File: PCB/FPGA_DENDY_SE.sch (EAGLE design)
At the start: 138 parts, among them CN1 DENDY60PINSLOT, J1 NTSC/PAL, J2 DENDY, Q1 14.318 MHz, Q2 17.734 MHz, U1 EP1C3T100C8N, U10 OPA2134U, U11 SN74LVC2G34DBVR, U12 THS7314DR, U13 74LS373WMSO20, U14 SN74LVC1G125DBVR, U15 74LVC1G04GV, U16 SN74LVC1G3157, U2 EPCS4, U3 SN74LVC8T245, U4 SN74LVC8T245, U5 SN74LVC1G240DBVR, U6 SN74LVC1G240DBVR, U7 SN74LVC1G240DBVR, U8 SN74LVC1G240DBVR, X1 057-010-1

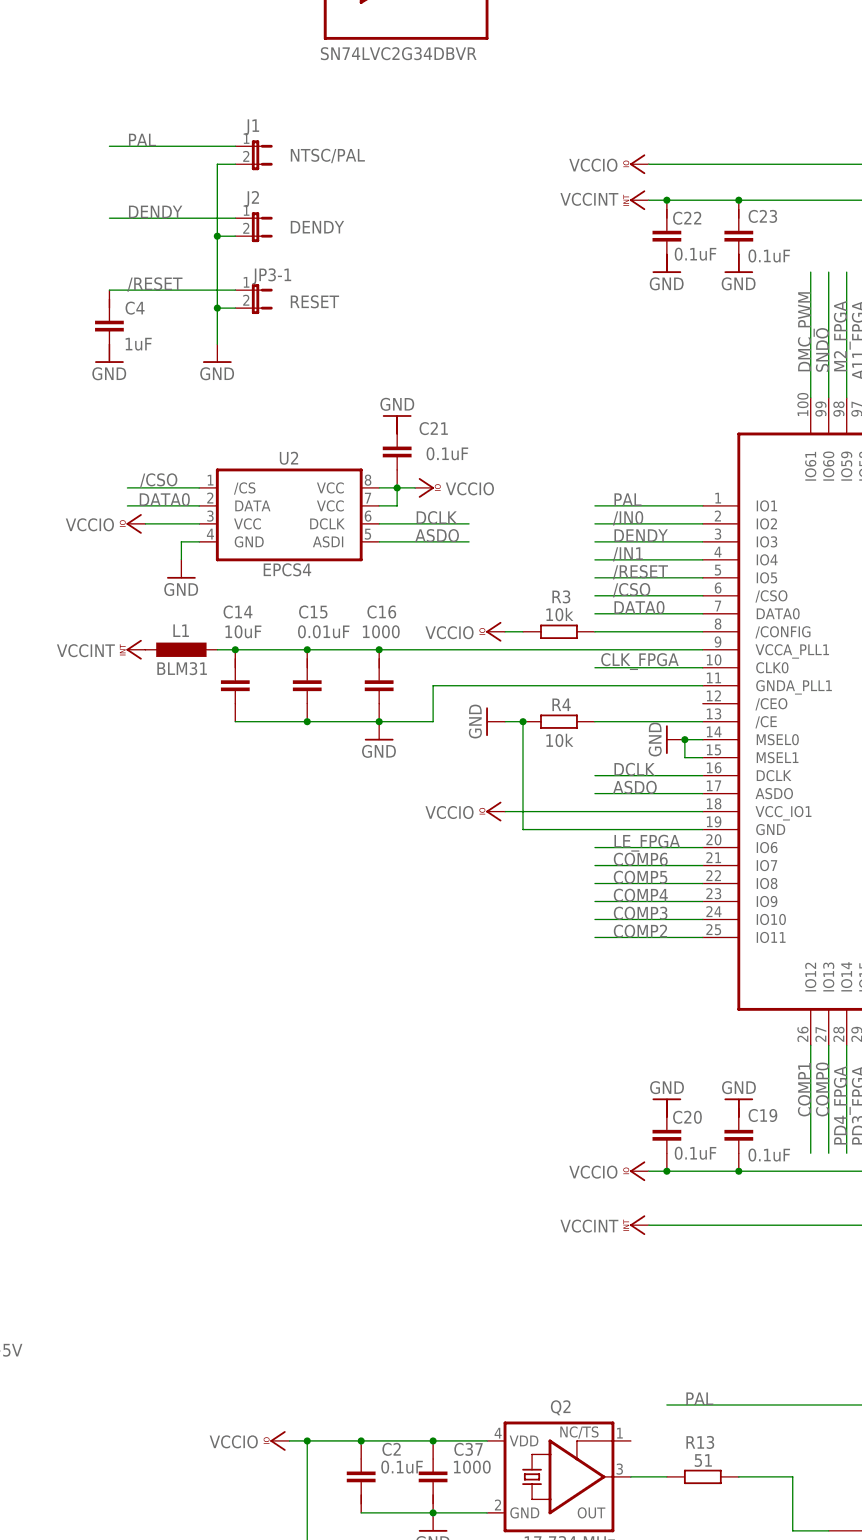
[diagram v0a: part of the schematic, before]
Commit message: Add files via upload
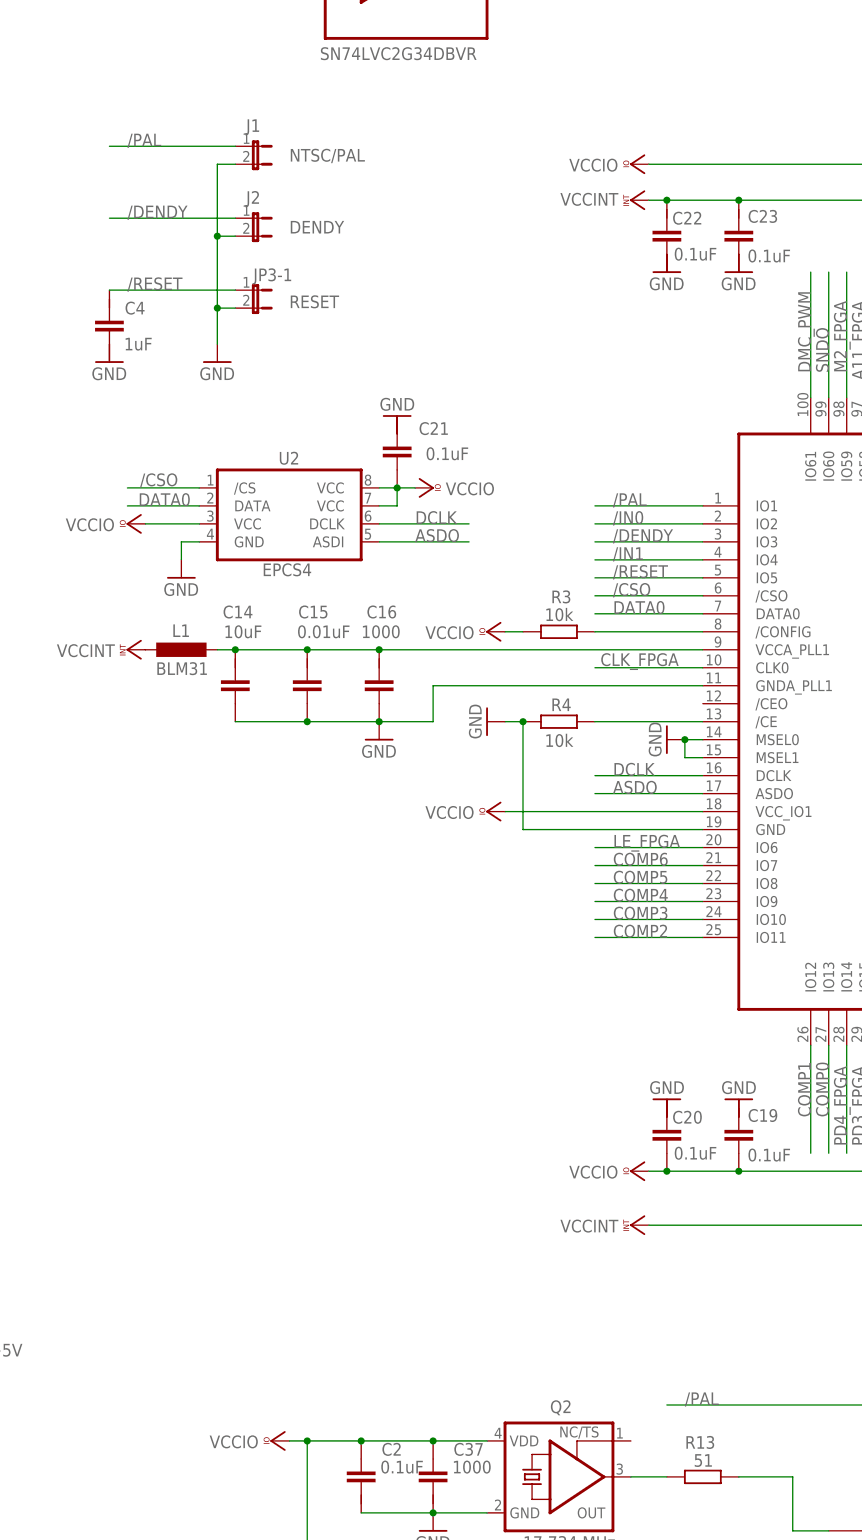
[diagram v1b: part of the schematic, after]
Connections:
- net DENDY renamed /DENDY
- net PAL renamed /PAL
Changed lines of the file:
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@@
-</segment>
-</net>
-<net name="DENDY" class="0">
-<segment>
-<pinref part="J2" gate="A" pin="1"/>
-<wire x1="-111.76" y1="68.58" x2="-129.54" y2="68.58" width="0.1524" layer="91"/>
-<label x="-127" y="68.58" size="1.778" layer="95"/>
-</segment>
-<segment>
-<wire x1="-45.72" y1="22.86" x2="-60.96" y2="22.86" width="0.1524" layer="91"/>
-<label x="-58.42" y="22.86" size="1.778" layer="95"/>
-<pinref part="U1" gate="G$1" pin="IO3"/>
 </segment>
 </net>
@@
 <pinref part="Q2" gate="G$1" pin="OUT"/>
 <wire x1="-50.8" y1="-109.22" x2="-55.88" y2="-109.22" width="0.1524" layer="91"/>
-</segment>
-</net>
-<net name="PAL" class="0">
-<segment>
-<pinref part="J1" gate="A" pin="1"/>
-<wire x1="-111.76" y1="78.74" x2="-129.54" y2="78.74" width="0.1524" layer="91"/>
-<label x="-127" y="78.74" size="1.778" layer="95"/>
-</segment>
-<segment>
-<wire x1="-45.72" y1="27.94" x2="-60.96" y2="27.94" width="0.1524" layer="91"/>
-<label x="-58.42" y="27.94" size="1.778" layer="95"/>
-<pinref part="U1" gate="G$1" pin="IO1"/>
-</segment>
-<segment>
-<wire x1="-17.78" y1="-99.06" x2="-50.8" y2="-99.06" width="0.1524" layer="91"/>
-<label x="-48.26" y="-99.06" size="1.778" layer="95"/>
-<pinref part="U16" gate="G$1" pin="S"/>
-<wire x1="-17.78" y1="-99.06" x2="-17.78" y2="-106.68" width="0.1524" layer="91"/>
 </segment>
 </net>
@@
 </segment>
 </net>
+<net name="/PAL" class="0">
+<segment>
+<pinref part="J1" gate="A" pin="1"/>
+<wire x1="-111.76" y1="78.74" x2="-129.54" y2="78.74" width="0.1524" layer="91"/>
+<label x="-127" y="78.74" size="1.778" layer="95"/>
+</segment>
+<segment>
+<wire x1="-45.72" y1="27.94" x2="-60.96" y2="27.94" width="0.1524" layer="91"/>
+<label x="-58.42" y="27.94" size="1.778" layer="95"/>
+<pinref part="U1" gate="G$1" pin="IO1"/>
+</segment>
+<segment>
+<wire x1="-17.78" y1="-99.06" x2="-50.8" y2="-99.06" width="0.1524" layer="91"/>
+<label x="-48.26" y="-99.06" size="1.778" layer="95"/>
+<pinref part="U16" gate="G$1" pin="S"/>
+<wire x1="-17.78" y1="-99.06" x2="-17.78" y2="-106.68" width="0.1524" layer="91"/>
+</segment>
+</net>
+<net name="/DENDY" class="0">
+<segment>
+<pinref part="J2" gate="A" pin="1"/>
+<wire x1="-111.76" y1="68.58" x2="-129.54" y2="68.58" width="0.1524" layer="91"/>
+<label x="-127" y="68.58" size="1.778" layer="95"/>
+</segment>
+<segment>
+<wire x1="-45.72" y1="22.86" x2="-60.96" y2="22.86" width="0.1524" layer="91"/>
+<label x="-58.42" y="22.86" size="1.778" layer="95"/>
+<pinref part="U1" gate="G$1" pin="IO3"/>
+</segment>
+</net>

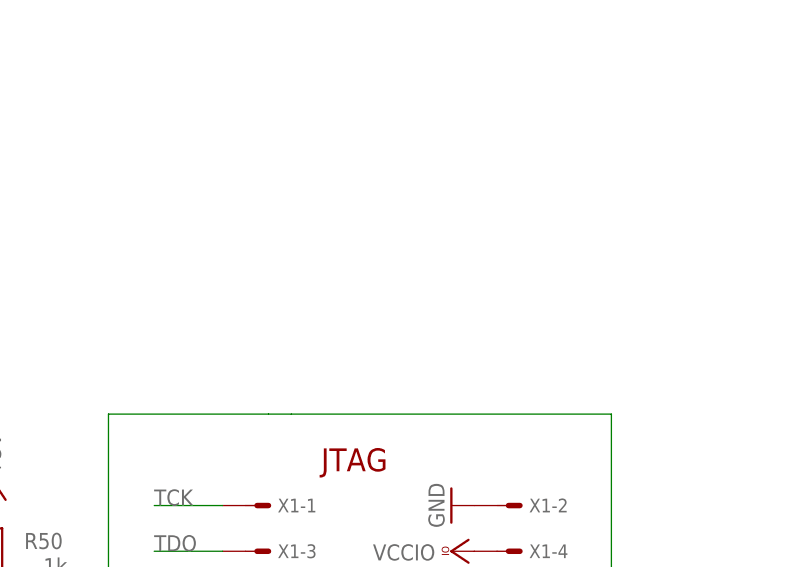
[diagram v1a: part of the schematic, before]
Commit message: Add files via upload
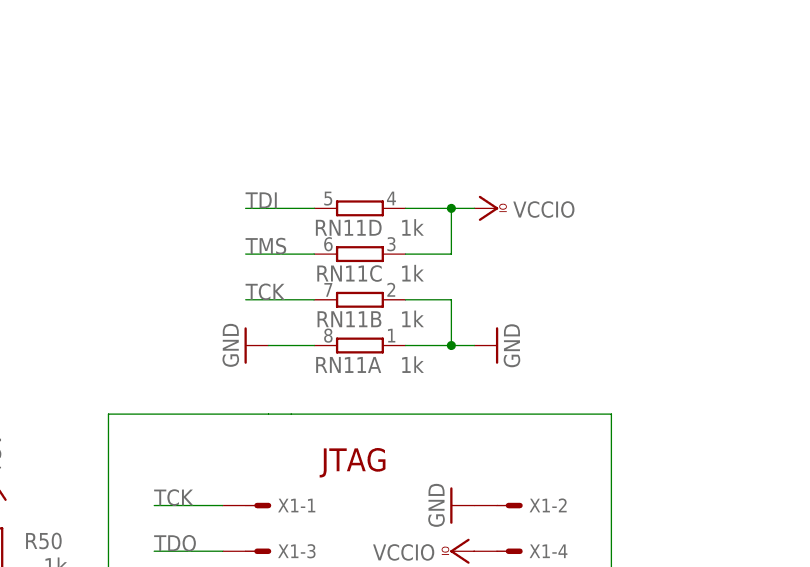
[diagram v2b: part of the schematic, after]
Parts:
- added RN11: 1k, resistor-dil:4R-N0603-ARC
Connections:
- net GND: now also RN11A.1, RN11A.2, RN11B.1
- net TCK: now also RN11B.2
- net TDI: now also RN11D.2
- net TMS: now also RN11C.2
- net VCCIO: now also RN11C.1, RN11D.1
